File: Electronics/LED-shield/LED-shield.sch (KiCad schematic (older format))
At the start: 31 parts, among them M1 ARDUINOUNO, U1 PCA9622

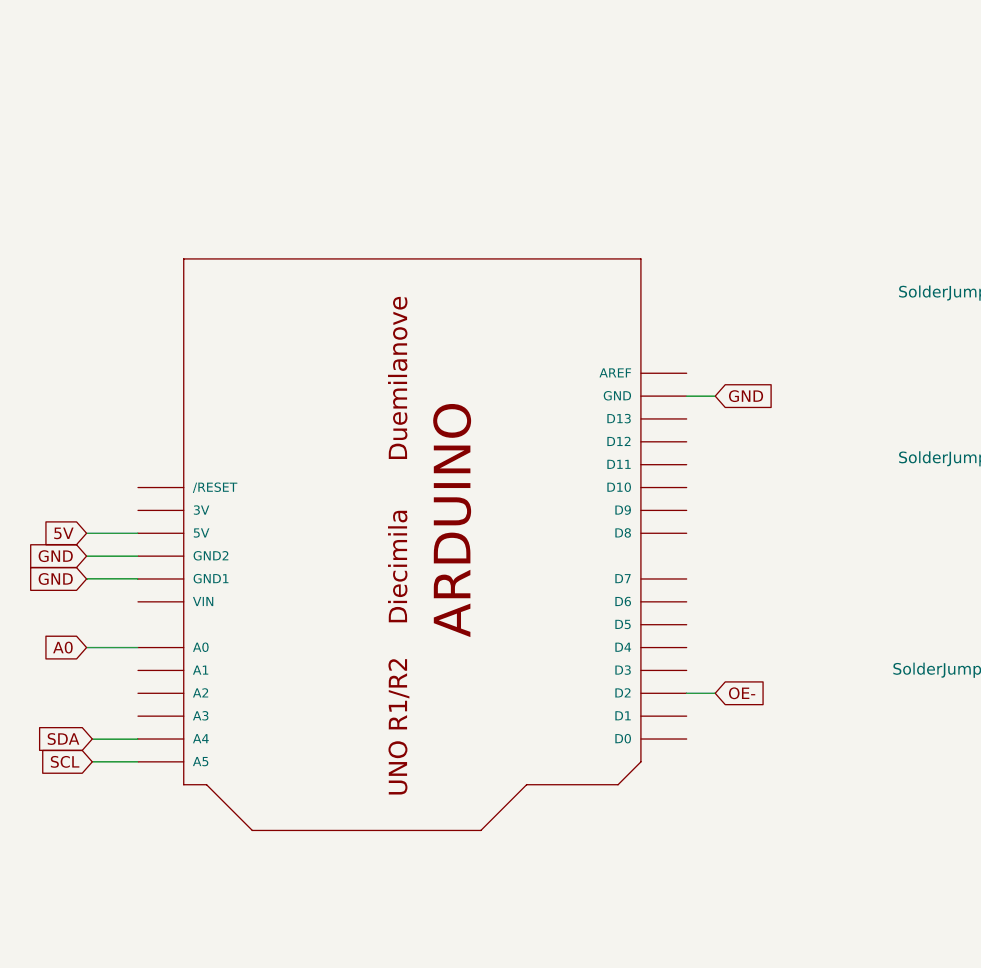
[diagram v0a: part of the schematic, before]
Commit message: Sally's shield design.
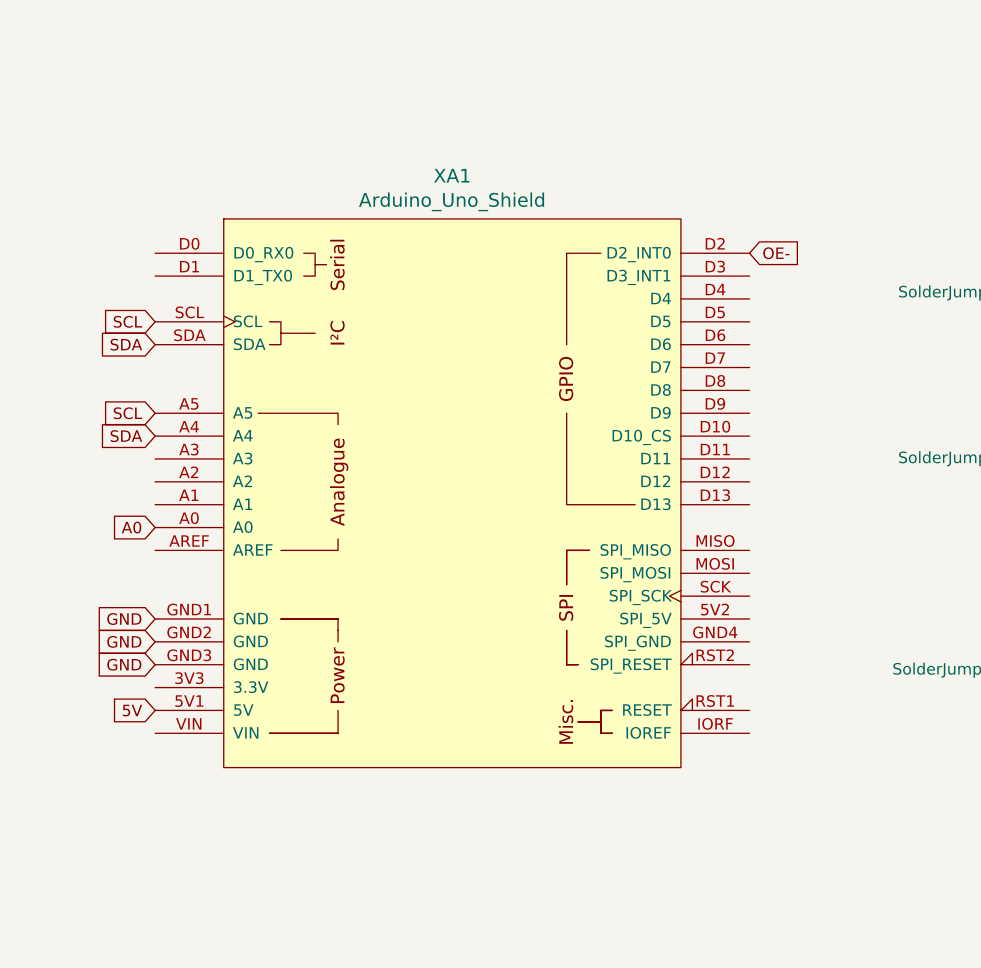
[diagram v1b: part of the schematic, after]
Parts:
- removed M1: ARDUINOUNO, adafruit-new_ARDUINO, symbol adafruit-new:ARDUINOUNO
- added XA1: Arduino_Uno_Shield, arduino:Arduino_Uno_Shield, symbol arduino:Arduino_Uno_Shield
- JP1, JP2, JP3: footprint (none) -> Jumper:SolderJumper-3_P1.3mm_Open_Pad1.0x1.5mm
- JP4, JP5: footprint adafruit-new_1X12 -> Connector_PinHeader_2.54mm:PinHeader_1x12_P2.54mm_Vertical
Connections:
- net 5V: now also XA1.5V1 (5V)
- net A0: now also XA1.A0
- net GND: now also XA1.GND1 (GND), XA1.GND2 (GND), XA1.GND3 (GND)
- net OE-: now also XA1.D2 (D2_INT0)
- net SCL: now also XA1.A5, XA1.SCL
- net SDA: now also XA1.A4, XA1.SDA
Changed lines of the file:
@@
 $EndDescr
-$Comp
-L adafruit-new:ARDUINOUNO M1
-U 1 1 5FABDAAC
-P 3500 3125
-F 0 "M1" H 3500 3125 45  0001 C CNN
-F 1 "ARDUINOUNO" H 3500 3125 45  0001 C CNN
-F 2 "adafruit-new_ARDUINO" H 3530 3275 20  0001 C CNN
-F 3 "" H 3500 3125 50  0001 C CNN
-	1    3500 3125
-	0    1    1    0
-$EndComp
-Text GLabel 1975 3425 0    50   Input ~ 0
-5V
-Text GLabel 1975 3525 0    50   Input ~ 0
-GND
-Text GLabel 1975 3625 0    50   Input ~ 0
-GND
-Text GLabel 4725 2825 2    50   Input ~ 0
-GND
-Text GLabel 2000 4325 0    50   Input ~ 0
-SDA
-Text GLabel 2000 4425 0    50   Input ~ 0
-SCL
-Wire Wire Line
-	1975 3425 2200 3425
-Wire Wire Line
-	2200 3525 1975 3525
-Wire Wire Line
-	1975 3625 2200 3625
-Wire Wire Line
-	2200 4325 2000 4325
-Wire Wire Line
-	2000 4425 2200 4425
-Wire Wire Line
-	4725 2825 4600 2825
 $Comp
 L reprapltd-kicad:PCA9622 U1
@@
 Wire Wire Line
 	7025 2425 6975 2425
-Text GLabel 4725 4125 2    50   Input ~ 0
-OE-
 Text GLabel 6925 2525 0    50   Input ~ 0
 OE-
 Wire Wire Line
 	7025 2525 6925 2525
-Wire Wire Line
-	4725 4125 4600 4125
 $Comp
 L Jumper:SolderJumper_3_Open JP2
@@
 F 0 "JP2" V 6396 2392 50  0000 L CNN
 F 1 "SolderJumper_3_Open" V 6305 2392 50  0000 L CNN
-F 2 "" H 6350 2325 50  0001 C CNN
+F 2 "Jumper:SolderJumper-3_P1.3mm_Open_Pad1.0x1.5mm" H 6350 2325 50  0001 C CNN
 F 3 "~" H 6350 2325 50  0001 C CNN
 	1    6350 2325
@@
 F 0 "JP3" V 6396 3117 50  0000 L CNN
 F 1 "SolderJumper_3_Open" V 6305 3117 50  0000 L CNN
-F 2 "" H 6350 3050 50  0001 C CNN
+F 2 "Jumper:SolderJumper-3_P1.3mm_Open_Pad1.0x1.5mm" H 6350 3050 50  0001 C CNN
 F 3 "~" H 6350 3050 50  0001 C CNN
 	1    6350 3050
@@
 F 0 "JP1" V 6371 4042 50  0000 L CNN
 F 1 "SolderJumper_3_Open" V 6280 4042 50  0000 L CNN
-F 2 "" H 6325 3975 50  0001 C CNN
+F 2 "Jumper:SolderJumper-3_P1.3mm_Open_Pad1.0x1.5mm" H 6325 3975 50  0001 C CNN
 F 3 "~" H 6325 3975 50  0001 C CNN
 	1    6325 3975
@@
 F 0 "JP4" V 8804 1500 45  0000 C CNN
 F 1 "PINHD-1X12" V 8720 1500 45  0000 C CNN
-F 2 "adafruit-new_1X12" H 8630 1700 20  0001 C CNN
+F 2 "Connector_PinHeader_2.54mm:PinHeader_1x12_P2.54mm_Vertical" H 8630 1700 20  0001 C CNN
 F 3 "" H 8600 1550 50  0001 C CNN
 	1    8600 1550
@@
 F 0 "JP5" V 9929 3675 45  0000 C CNN
 F 1 "PINHD-1X12" V 9845 3675 45  0000 C CNN
-F 2 "adafruit-new_1X12" H 9755 3875 20  0001 C CNN
+F 2 "Connector_PinHeader_2.54mm:PinHeader_1x12_P2.54mm_Vertical" H 9755 3875 20  0001 C CNN
 F 3 "" H 9725 3725 50  0001 C CNN
 	1    9725 3725
@@
 Text GLabel 10225 4825 3    50   Input ~ 0
 GND
-Text GLabel 1975 3925 0    50   Input ~ 0
-A0
-Wire Wire Line
-	2200 3925 1975 3925
 Text GLabel 9425 1400 1    50   Input ~ 0
 A0
@@
 Wire Wire Line
 	8950 1450 8950 1400
+$Comp
+L arduino:Arduino_Uno_Shield XA1
+U 1 1 605A7BB6
+P 3575 3250
+F 0 "XA1" H 3575 4637 60  0000 C CNN
+F 1 "Arduino_Uno_Shield" H 3575 4531 60  0000 C CNN
+F 2 "arduino:Arduino_Uno_Shield" H 5375 7000 60  0001 C CNN
+F 3 "https://store.arduino.cc/arduino-uno-rev3" H 5375 7000 60  0001 C CNN
+	1    3575 3250
+	1    0    0    -1
+$EndComp
+Text GLabel 4875 2200 2    50   Input ~ 0
+OE-
+Text GLabel 2275 3800 0    50   Input ~ 0
+GND
+Text GLabel 2275 3900 0    50   Input ~ 0
+GND
+Text GLabel 2275 4000 0    50   Input ~ 0
+GND
+Text GLabel 2275 2500 0    50   Input ~ 0
+SCL
+Text GLabel 2275 2600 0    50   Input ~ 0
+SDA
+Text GLabel 2275 3400 0    50   Input ~ 0
+A0
+Text GLabel 2275 4200 0    50   Input ~ 0
+5V
+Text GLabel 2275 3000 0    50   Input ~ 0
+SDA
+Text GLabel 2275 2900 0    50   Input ~ 0
+SCL
 $EndSCHEMATC
